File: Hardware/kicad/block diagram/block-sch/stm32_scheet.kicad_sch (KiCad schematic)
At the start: 18 parts, among them Q2 BC817, SW1 Power Button, U6 STM32L4Q5, Y1 Crystal

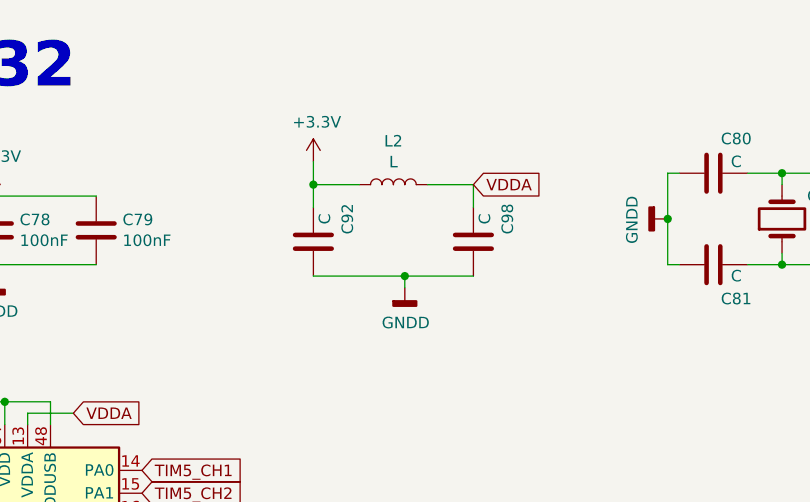
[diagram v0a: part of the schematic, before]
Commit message: new
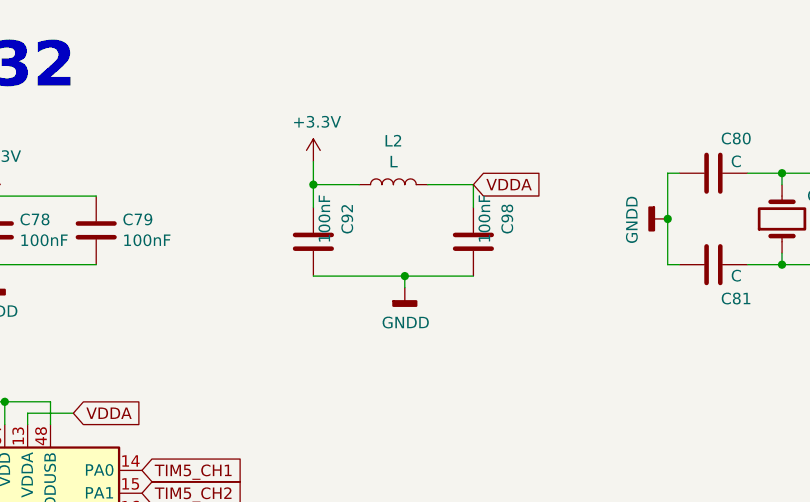
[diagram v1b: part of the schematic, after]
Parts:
- C80, C81, C82: footprint Capacitor_SMD:C_1206_3216Metric -> Capacitor_SMD:C_0805_2012Metric
- C92, C98: value C -> 100nF; footprint Capacitor_SMD:C_1206_3216Metric -> Capacitor_SMD:C_0805_2012Metric
- D9: footprint LED_SMD:LED_1206_3216Metric -> LED_SMD:LED_0805_2012Metric
- L1, L2: footprint Inductor_SMD:L_1206_3216Metric -> Inductor_SMD:L_0805_2012Metric
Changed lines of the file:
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@@
     (in_bom yes) (on_board yes)
     (property "Reference" "C92" (id 0) (at 95.25 36.83 90))
-    (property "Value" "C" (id 1) (at 92.71 36.83 90))
-    (property "Footprint" "Capacitor_SMD:C_1206_3216Metric" (id 2) (at 90.4748 35.56 0)
+    (property "Value" "100nF" (id 1) (at 92.71 36.83 90))
+    (property "Footprint" "Capacitor_SMD:C_0805_2012Metric" (id 2) (at 90.4748 35.56 0)
       (effects (font (size 1.27 1.27)) hide)
     )
@@
     (in_bom yes) (on_board yes)
     (property "Reference" "C98" (id 0) (at 113.03 36.83 90))
-    (property "Value" "C" (id 1) (at 110.49 36.83 90))
-    (property "Footprint" "Capacitor_SMD:C_1206_3216Metric" (id 2) (at 108.2548 35.56 0)
+    (property "Value" "100nF" (id 1) (at 110.49 36.83 90))
+    (property "Footprint" "Capacitor_SMD:C_0805_2012Metric" (id 2) (at 108.2548 35.56 0)
       (effects (font (size 1.27 1.27)) hide)
     )
@@
     (property "Reference" "L2" (id 0) (at 100.33 28.194 90))
     (property "Value" "L" (id 1) (at 100.33 30.5054 90))
-    (property "Footprint" "Inductor_SMD:L_1206_3216Metric" (id 2) (at 100.33 33.02 0)
+    (property "Footprint" "Inductor_SMD:L_0805_2012Metric" (id 2) (at 100.33 33.02 0)
       (effects (font (size 1.27 1.27)) hide)
     )
@@
       (effects (font (size 1.27 1.27)) (justify left))
     )
-    (property "Footprint" "Inductor_SMD:L_1206_3216Metric" (id 2) (at 59.69 154.94 0)
+    (property "Footprint" "Inductor_SMD:L_0805_2012Metric" (id 2) (at 59.69 154.94 0)
       (effects (font (size 1.27 1.27)) hide)
     )
@@
     (property "Reference" "C81" (id 0) (at 138.43 45.72 90))
     (property "Value" "C" (id 1) (at 138.43 43.18 90))
-    (property "Footprint" "Capacitor_SMD:C_1206_3216Metric" (id 2) (at 139.7 40.9448 0)
+    (property "Footprint" "Capacitor_SMD:C_0805_2012Metric" (id 2) (at 139.7 40.9448 0)
       (effects (font (size 1.27 1.27)) hide)
     )
@@
     (property "Reference" "C80" (id 0) (at 138.43 27.94 90))
     (property "Value" "C" (id 1) (at 138.43 30.48 90))
-    (property "Footprint" "Capacitor_SMD:C_1206_3216Metric" (id 2) (at 139.7 30.7848 0)
+    (property "Footprint" "Capacitor_SMD:C_0805_2012Metric" (id 2) (at 139.7 30.7848 0)
       (effects (font (size 1.27 1.27)) hide)
     )
@@
       (effects (font (size 1.27 1.27)) (justify right))
     )
-    (property "Footprint" "LED_SMD:LED_1206_3216Metric" (id 2) (at 271.78 143.51 0)
+    (property "Footprint" "LED_SMD:LED_0805_2012Metric" (id 2) (at 271.78 143.51 0)
       (effects (font (size 1.27 1.27)) hide)
     )
@@
       (effects (font (size 1.27 1.27)) (justify left))
     )
-    (property "Footprint" "Capacitor_SMD:C_1206_3216Metric" (id 2) (at 230.8352 160.02 0)
-      (effects (font (size 1.27 1.27)) hide)
-    )
+    (property "Footprint" "Capacitor_SMD:C_0805_2012Metric" (id 2) (at 230.8352 160.02 0)
+      (effects (font (size 1.27 1.27)) hide)
+    )

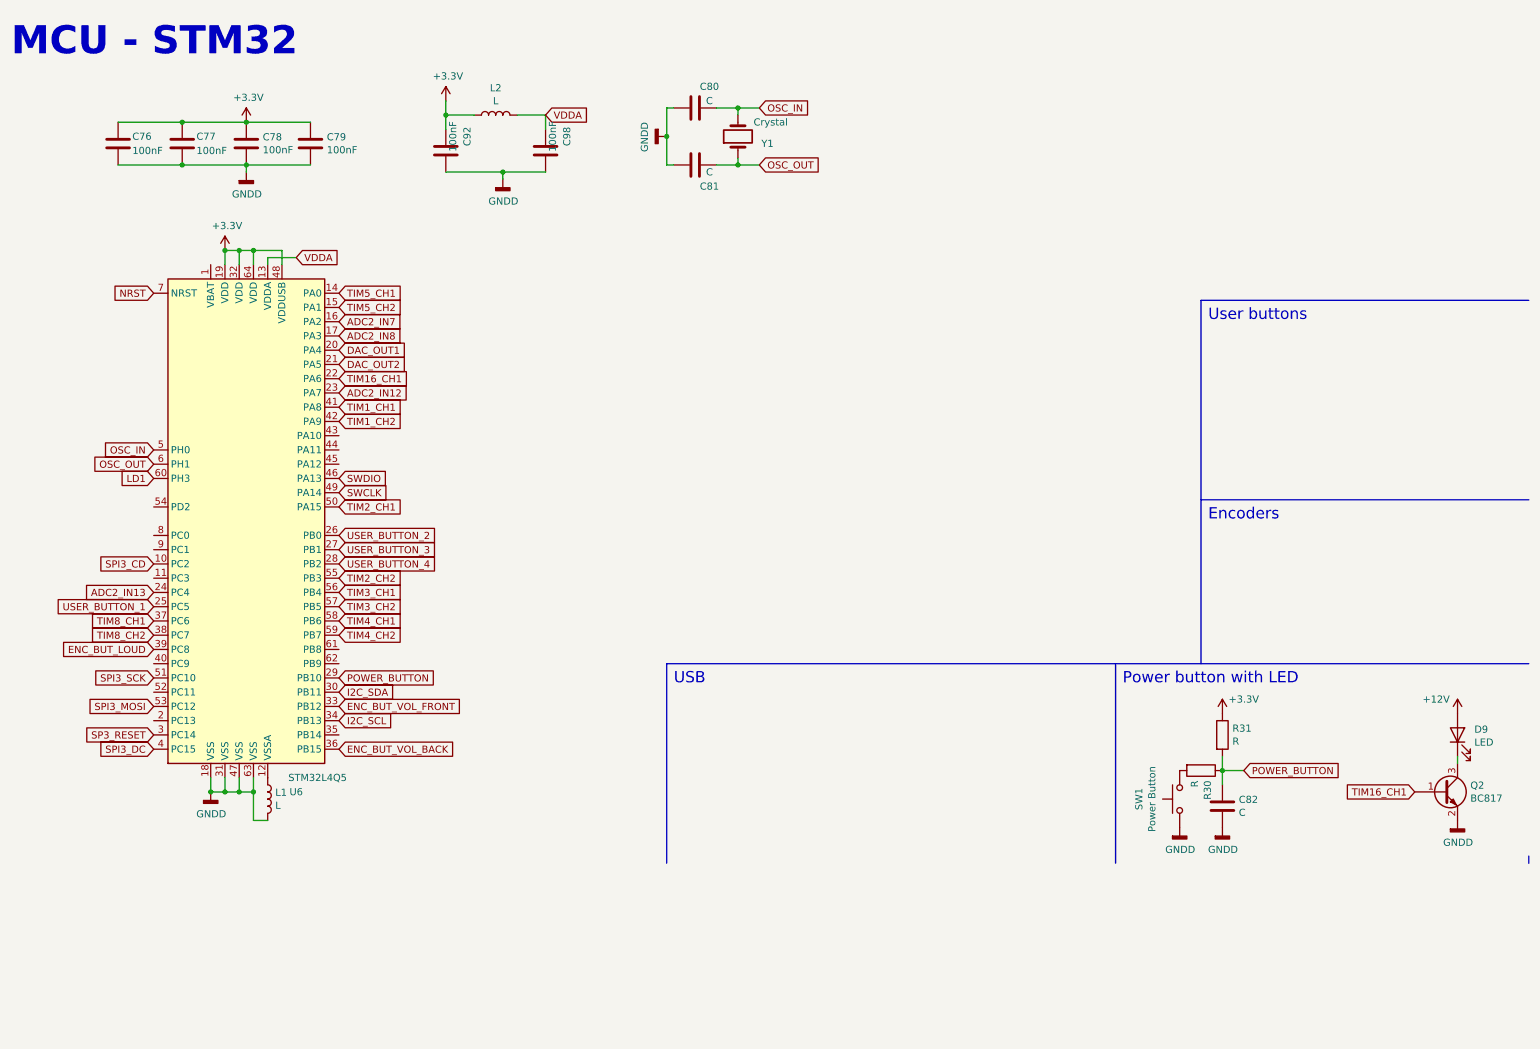
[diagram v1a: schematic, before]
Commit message: new
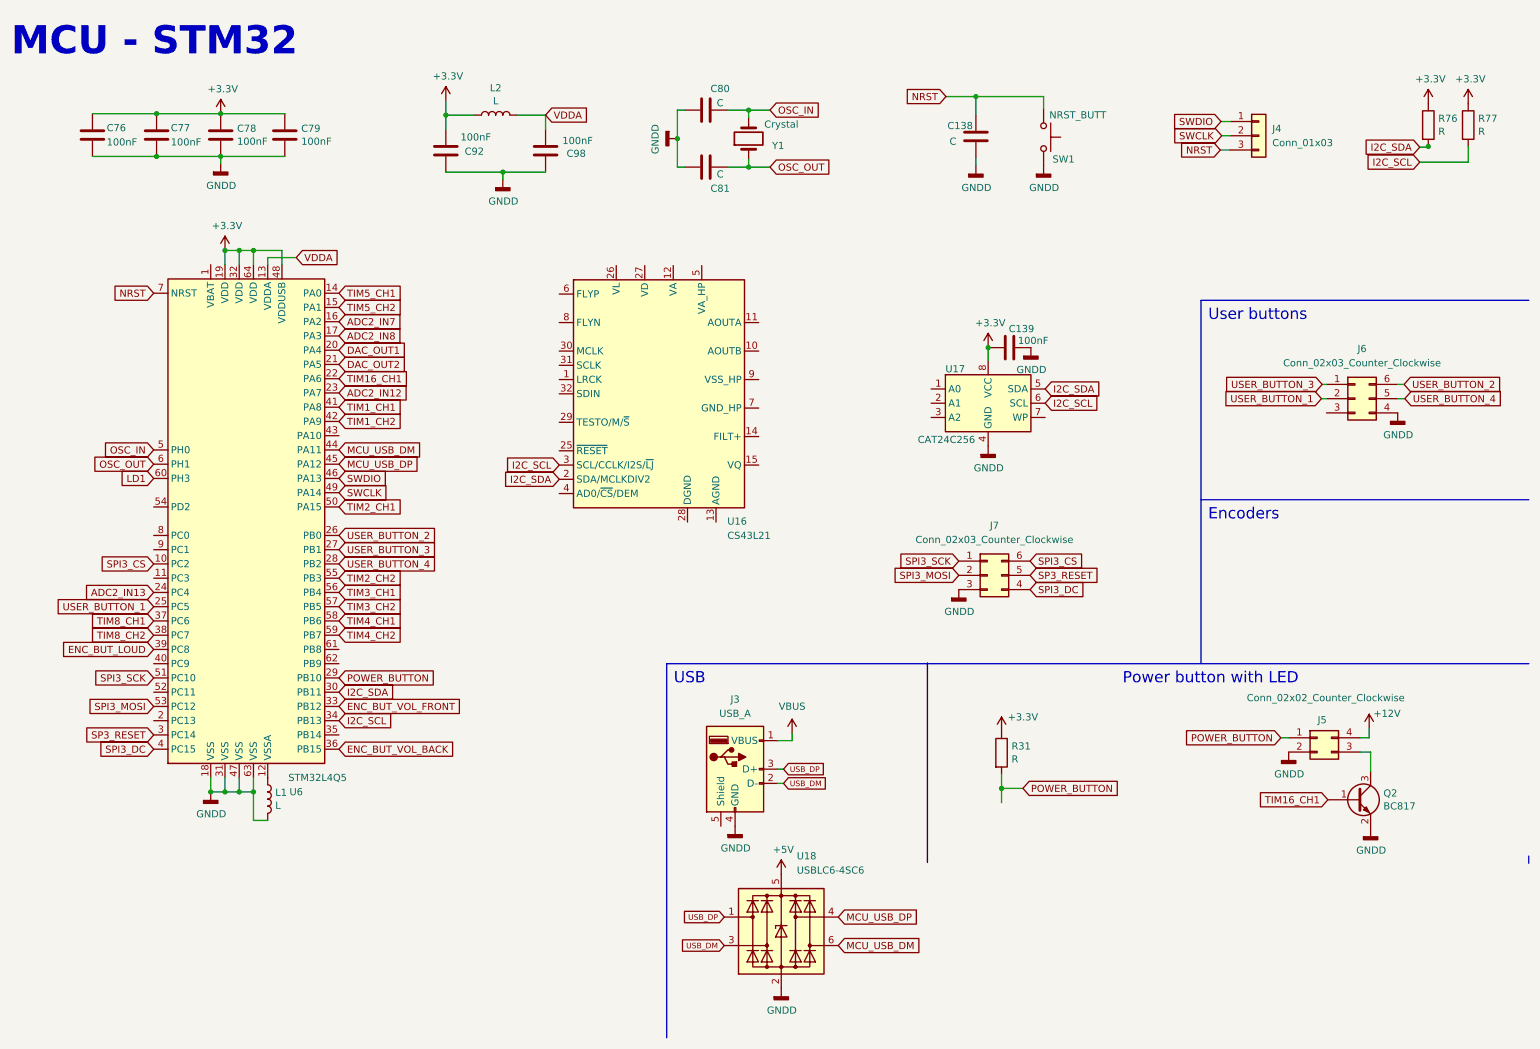
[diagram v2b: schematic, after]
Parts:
- removed C82: C, Capacitor_SMD:C_0805_2012Metric, symbol Device:C
- removed D9: LED, LED_SMD:LED_0805_2012Metric, symbol Device:LED
- removed R30: R, Resistor_SMD:R_1206_3216Metric, symbol Device:R
- added C138: C, Capacitor_SMD:C_0805_2012Metric, symbol Device:C
- added C139: 100nF, Capacitor_SMD:C_0805_2012Metric, symbol Device:C
- added J3: USB_A, amplituner_lib:usb_A, symbol Connector:USB_A
- added J4: Conn_01x03, Connector_PinHeader_2.54mm:PinHeader_1x03_P2.54mm_Vertical, symbol Connector_Generic:Conn_01x03
- added J5: Conn_02x02_Counter_Clockwise, Connector_PinHeader_2.54mm:PinHeader_2x02_P2.54mm_Vertical, symbol Connector_Generic:Conn_02x02_Counter_Clockwise
- added J6, J7: Conn_02x03_Counter_Clockwise, Connector_PinHeader_2.54mm:PinHeader_2x03_P2.54mm_Vertical, symbol Connector_Generic:Conn_02x03_Counter_Clockwise
- added R76, R77: R, Resistor_SMD:R_1206_3216Metric, symbol Device:R
- added U16: CS43L21, Package_DFN_QFN:QFN-32-1EP_5x5mm_P0.5mm_EP3.45x3.45mm, symbol Audio:CS43L21
- added U17: CAT24C256, amplituner_lib:CAT24C256, symbol Memory_EEPROM:CAT24C256
- added U18: USBLC6-4SC6, Package_TO_SOT_SMD:SOT-23-6, symbol Power_Protection:USBLC6-4SC6
- SW1: value Power Button -> NRST_BUTT; footprint (none) -> Button_Switch_SMD:SW_SPST_FSMSM
- Y1: footprint Crystal:Crystal_HC52-6mm_Vertical -> Crystal:Crystal_SMD_HC49-SD
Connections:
- net +12V: now also J5.4 (Pin_4)
- net +3V3: now also C139.2, R76.1, R77.1, U17.8 (VCC)
- net GNDD: now also SW1.2, C138.2, C139.1, J3.4 (GND), J5.2 (Pin_2), J6.4 (Pin_4), J7.3 (Pin_3), U17.4 (GND), U18.2 (GND); no longer SW1.1
- net I2C_SCL: now also R77.2, U16.3 (SCL/CCLK/I2S/~{LJ}), U17.6 (SCL)
- net I2C_SDA: now also R76.2, U16.2 (SDA/MCLKDIV2), U17.5 (SDA)
- net NRST: now also SW1.1, C138.1, J4.3 (Pin_3)
- net POWER_BUTTON: now also J5.1 (Pin_1)
- net SP3_RESET: now also J7.5 (Pin_5)
- net SPI3_DC: now also J7.4 (Pin_4)
- net SPI3_MOSI: now also J7.2 (Pin_2)
- net SPI3_SCK: now also J7.1 (Pin_1)
- net SWCLK: now also J4.2 (Pin_2)
- net SWDIO: now also J4.1 (Pin_1)
- net USER_BUTTON_1: now also J6.2 (Pin_2)
- net USER_BUTTON_2: now also J6.6 (Pin_6)
- net USER_BUTTON_3: now also J6.1 (Pin_1)
- net USER_BUTTON_4: now also J6.5 (Pin_5)
- net MCU_USB_DM: now reaches U6.44 (PA11)
- net MCU_USB_DM: now also U18.6 (I/O4)
- net MCU_USB_DP: now reaches U6.45 (PA12)
- net MCU_USB_DP: now also U18.4 (I/O3)
- net at Q2.3 (C): now also J5.3 (Pin_3)
- net SPI3_CD renamed SPI3_CS
- net SPI3_CS: now also J7.6 (Pin_6)
- new net: U16.13 (AGND), U16.33 (AGND)
- new net +5V: U18.5 (VBUS)
- new net USB_DM: J3.2 (D-), U18.3 (I/O2)
- new net USB_DP: J3.3 (D+), U18.1 (I/O1)
- new net VBUS: J3.1 (VBUS)
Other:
- moved on the sheet: C76, C77, C78, C79, C80, C81, Q2, R31, Y1

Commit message: new
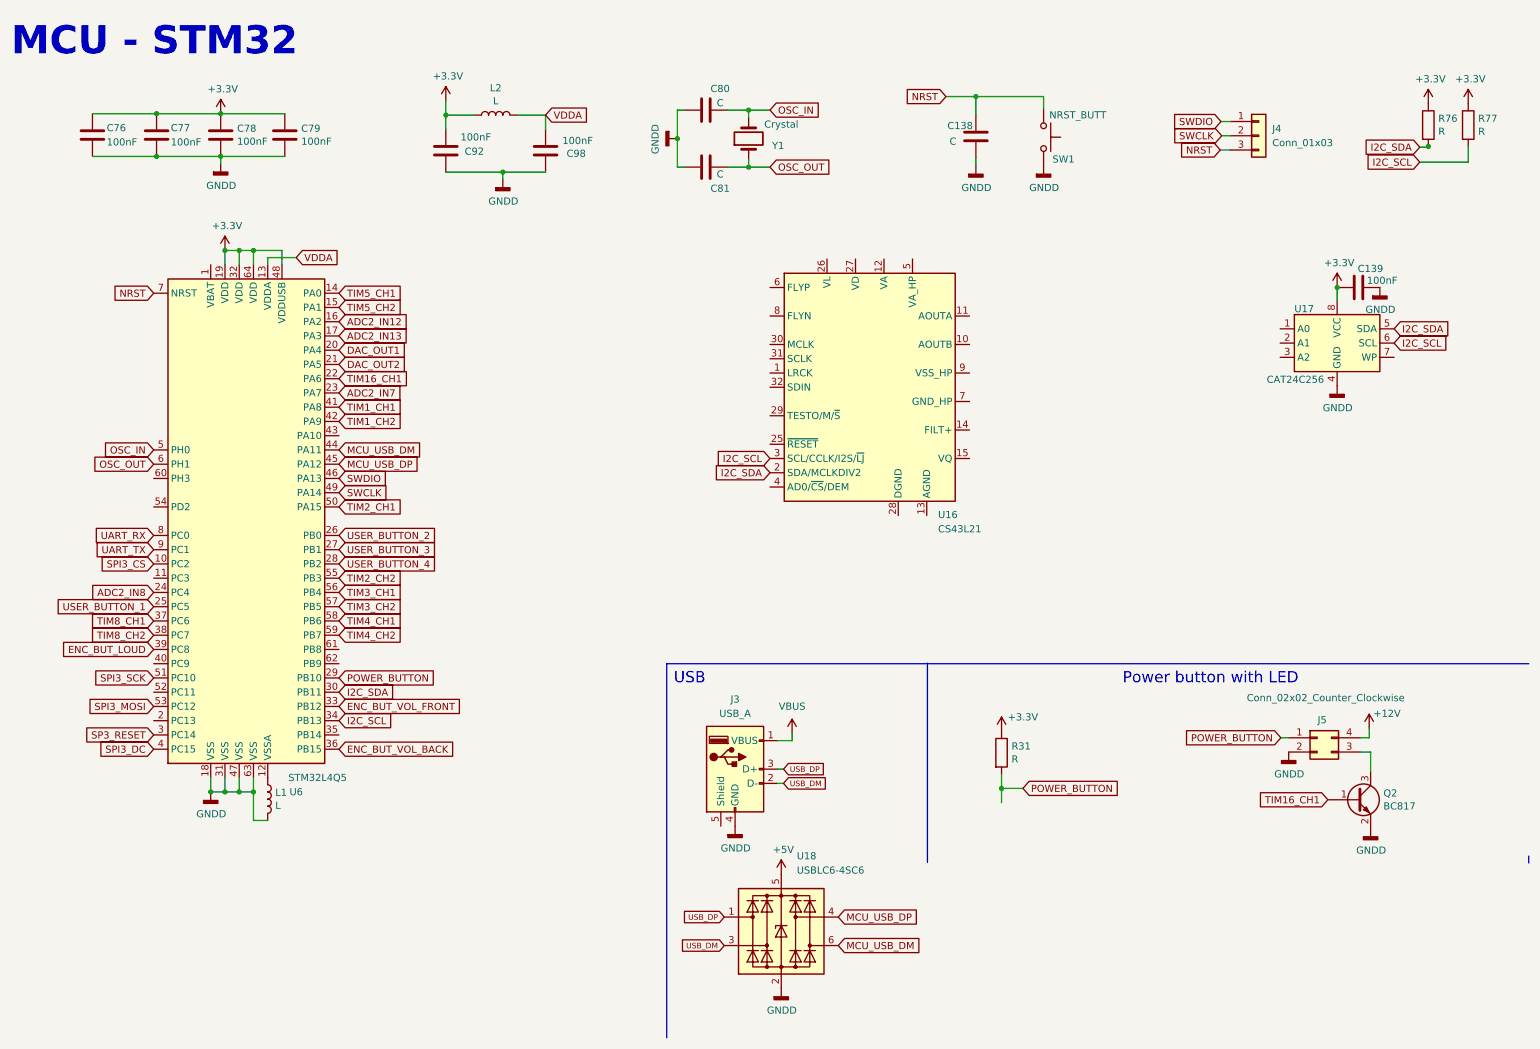
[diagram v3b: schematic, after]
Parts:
- removed J6, J7: Conn_02x03_Counter_Clockwise, Connector_PinHeader_2.54mm:PinHeader_2x03_P2.54mm_Vertical, symbol Connector_Generic:Conn_02x03_Counter_Clockwise
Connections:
- net ADC2_IN12: now also U6.16 (PA2); no longer U6.23 (PA7)
- net ADC2_IN13: now also U6.17 (PA3); no longer U6.24 (PC4)
- net ADC2_IN7: now also U6.23 (PA7); no longer U6.16 (PA2)
- net ADC2_IN8: now also U6.24 (PC4); no longer U6.17 (PA3)
- net UART_RX: now reaches U6.8 (PC0)
- net UART_TX: now reaches U6.9 (PC1)
- net LD1: no longer names the net of U6.60 (PH3)
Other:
- note removed: "Encoders"
- note removed: "User buttons"
- moved on the sheet: C139, U16, U17
